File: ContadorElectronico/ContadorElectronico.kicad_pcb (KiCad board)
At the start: 2 copper layers, 60 x 90 mm, 24 parts, among them J1 INPUT, J2 POWER, SW1 MODE, SW2 INC, SW3 DEC, U1 LM358, U3 4N35, U4 4N35

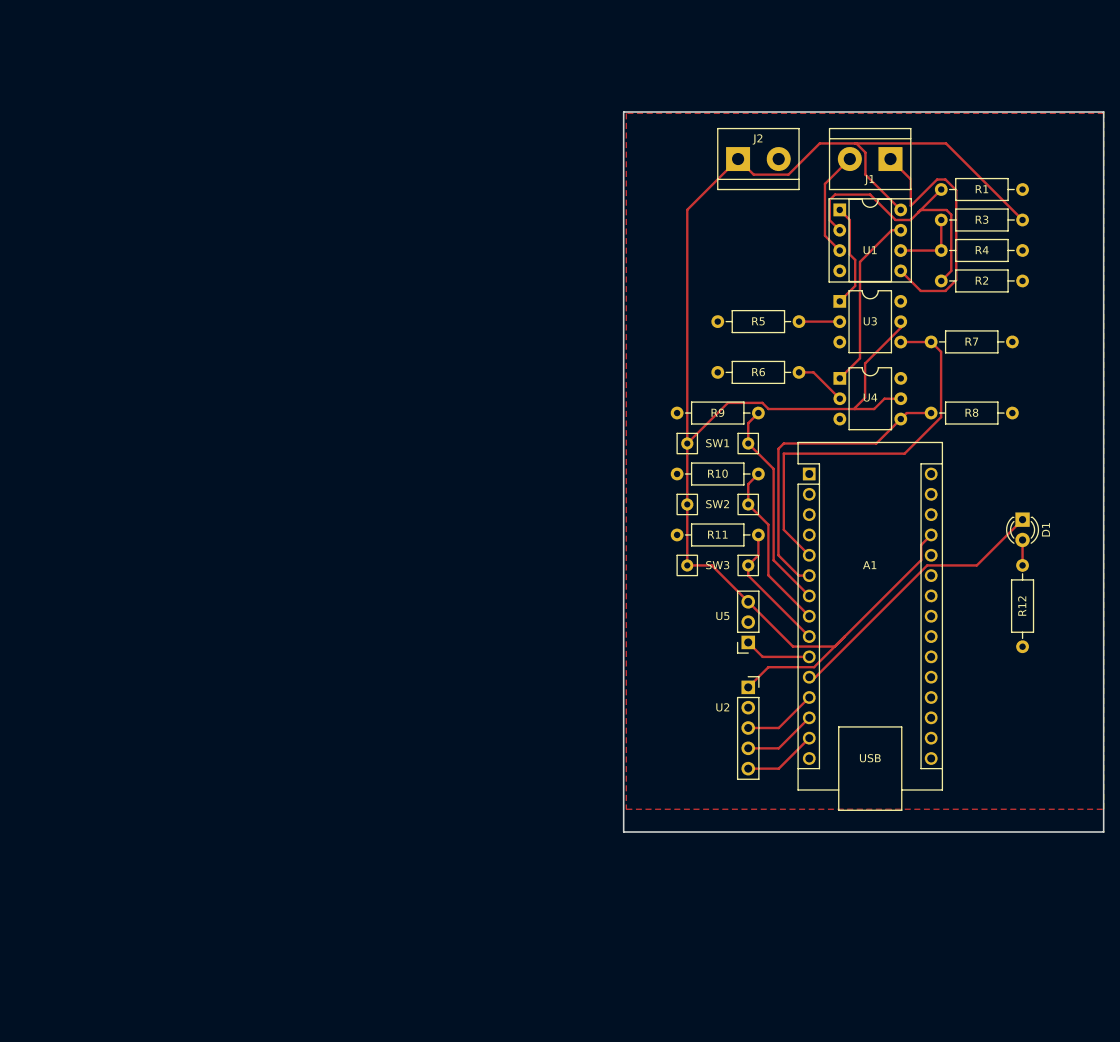
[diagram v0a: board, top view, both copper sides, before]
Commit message: Diseño inicial
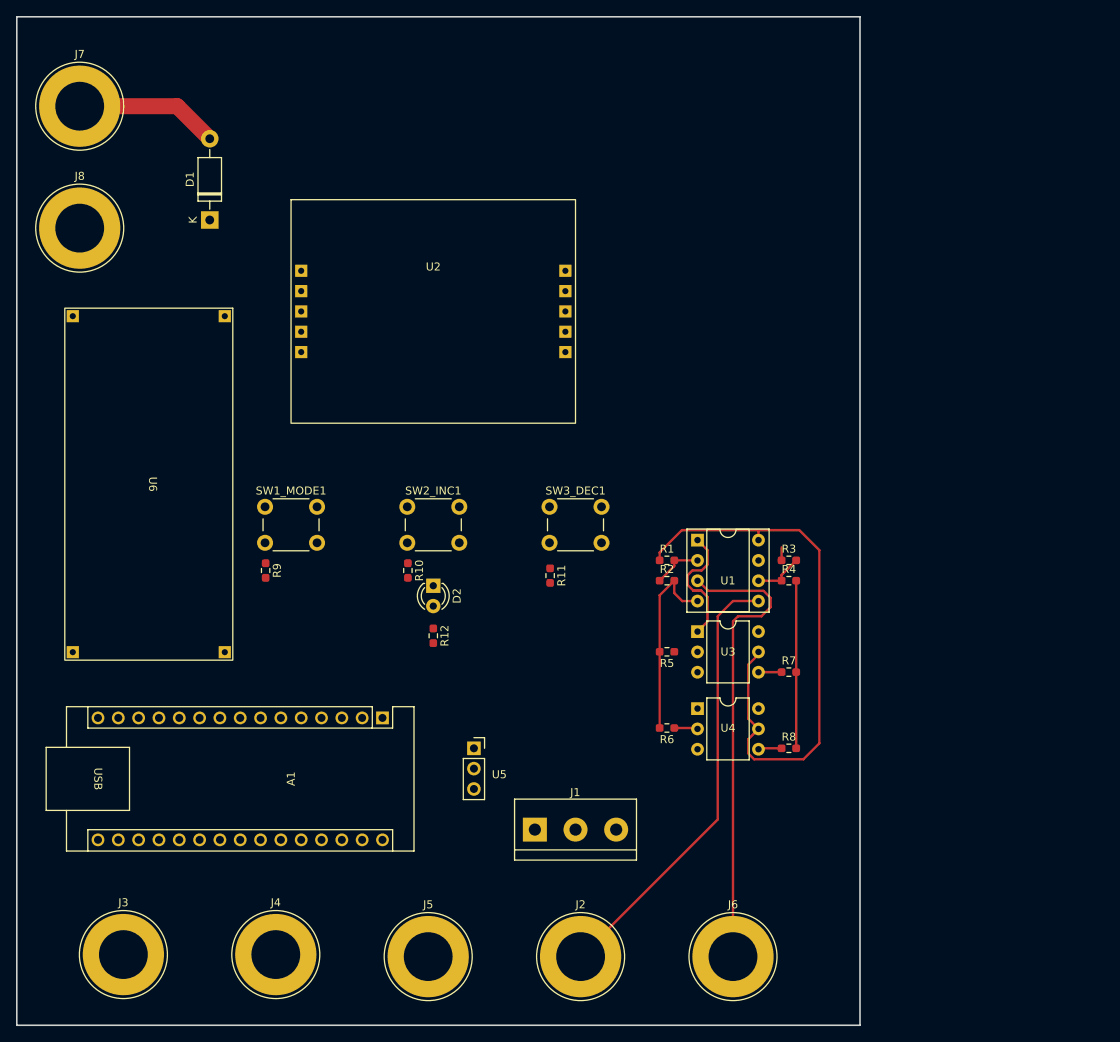
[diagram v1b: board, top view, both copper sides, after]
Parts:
- added D1: 1N4002, Diode_THT:D_DO-41_SOD81_P10.16mm_Horizontal, F.Cu at (48.3, 63.5)
- added J3: Conn_01x01_Pin, Connector:Banana_Jack_1Pin, F.Cu at (37.5, 155.3)
- added J4: Conn_01x01_Pin, Connector:Banana_Jack_1Pin, F.Cu at (56.5, 155.3)
- added J5: Conn_01x01_Pin, Connector:Banana_Jack_1Pin, F.Cu at (75.6, 155.6)
- added J6: Conn_01x01_Pin, Connector:Banana_Jack_1Pin, F.Cu at (113.7, 155.6)
- added J7: Conn_01x01_Pin, Connector:Banana_Jack_1Pin, F.Cu at (32.0, 49.3)
- added J8: Conn_01x01_Pin, Connector:Banana_Jack_1Pin, F.Cu at (32.0, 64.5)
- added U6: ~, Custom:LM2596 MODULE, F.Cu at (40.6, 96.5)
- J1: value INPUT -> Screw_Terminal_01x03; footprint TerminalBlock:TerminalBlock_bornier-2_P5.08mm -> TerminalBlock:TerminalBlock_bornier-3_P5.08mm
- J2: value POWER -> Conn_01x01_Pin; footprint TerminalBlock:TerminalBlock_bornier-2_P5.08mm -> Connector:Banana_Jack_1Pin
- R1, R10, R11, R12, R2, R3, R4, R5, R6, R7, R8, R9: footprint Resistor_THT:R_Axial_DIN0207_L6.3mm_D2.5mm_P10.16mm_Horizontal -> Resistor_SMD:R_0603_1608Metric_Pad0.98x0.95mm_HandSolder
- SW1_MODE1: renamed from SW1; footprint Custom:SW Header -> Button_Switch_THT:SW_PUSH_6mm
- SW2_INC1: renamed from SW2; footprint Custom:SW Header -> Button_Switch_THT:SW_PUSH_6mm
- SW3_DEC1: renamed from SW3; footprint Custom:SW Header -> Button_Switch_THT:SW_PUSH_6mm
- U2: footprint Connector_PinSocket_2.54mm:PinSocket_1x05_P2.54mm_Vertical -> Custom:2Digit7SEG
- moved J2 101.6 mm to (94.6, 155.6)
- moved J1 94.9 mm to (88.9, 139.7), turned to 0 degrees
- moved R12 74.2 mm to (76.2, 115.5)
- moved D2 74.1 mm to (76.2, 109.2)
- moved U2 65.3 mm to (76.2, 69.8)
- moved R9 64.7 mm to (55.2, 107.3), turned to -90 degrees
- moved R1 64.2 mm to (105.4, 106.0), turned to 0 degrees
- moved A1 61.4 mm to (69.8, 125.7), turned to -90 degrees
- moved SW1_MODE1 57.1 mm to (55.2, 99.3)
- moved R3 51.6 mm to (120.7, 106.0), turned to 0 degrees
- moved R2 50.8 mm to (105.4, 108.6)
- moved R6 47.4 mm to (105.4, 127.0)
- moved R8 45.5 mm to (120.7, 129.5)
- moved R4 45.5 mm to (120.7, 108.6)
- moved R10 45.4 mm to (73.0, 107.3), turned to -90 degrees
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- renumbered D1 to D2
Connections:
- A1 pad 30: unconnected-(A1-VIN-Pad30) -> +9V
- J1 pad 1: /RESET_IN -> /NC
- J1 pad 2: /COUNT_IN -> /COM
- J2 pad 1: +5V -> /RESET_IN
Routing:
- net +5V: track 205.4 -> 74.8 mm
- net /COUNT: track 49.3 -> 2.89 mm
- net /COUNT_IN: track 13.5 -> 58.5 mm
- net GND: track 0.00 -> 45.0 mm
- net /RESET: track 39.1 -> 2.93 mm
- net /MODE_LED: track 34.8 -> 0.00 mm
- net Net-(U1A--): track 34.7 -> 6.21 mm
- net /MODE: track 26.5 -> 0.00 mm
- net Net-(U1-Pad7): track 22.3 -> 0.00 mm
- net /INC: track 21.5 -> 0.00 mm
- net /RESET_IN: track 34.3 -> 55.5 mm
- net +24V: track 0.00 -> 17.9 mm
- net /DEC: track 16.4 -> 0.00 mm
- net Net-(A1-D9): track 9.21 -> 0.00 mm
- net Net-(A1-D11): track 9.21 -> 0.00 mm
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- removed copper zone on F.Cu, net GND
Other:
- board size 60 x 90 mm -> 105.4 x 126.1 mm
